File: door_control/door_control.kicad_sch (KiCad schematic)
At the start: 27 parts

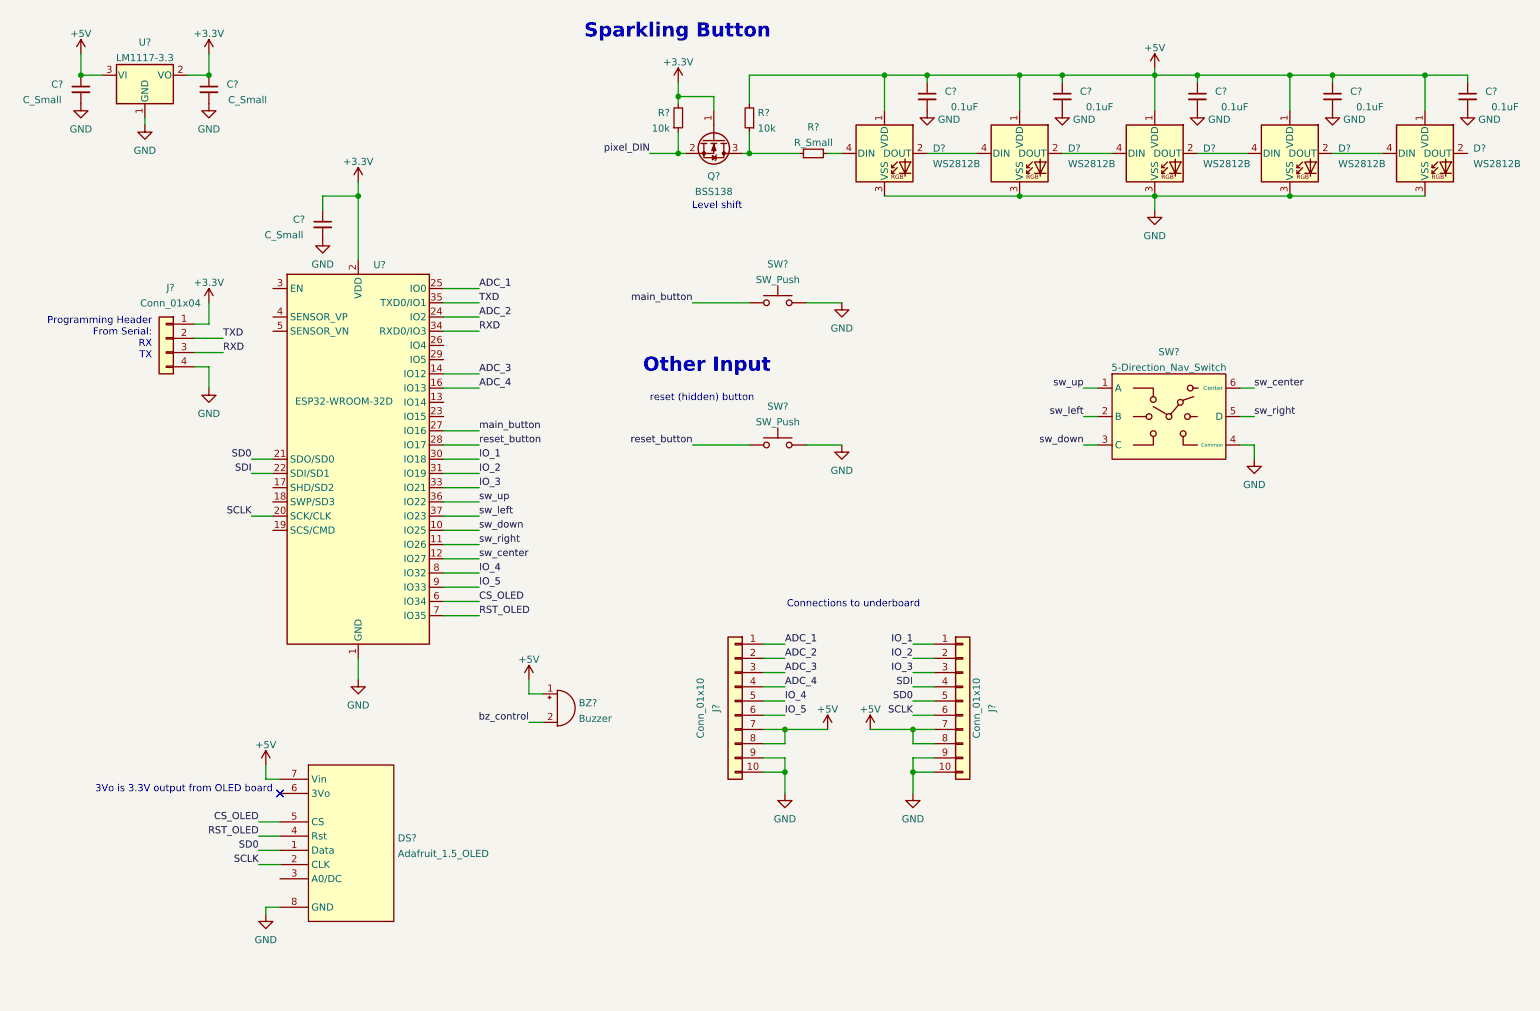
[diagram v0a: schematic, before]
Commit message: door control schematic update
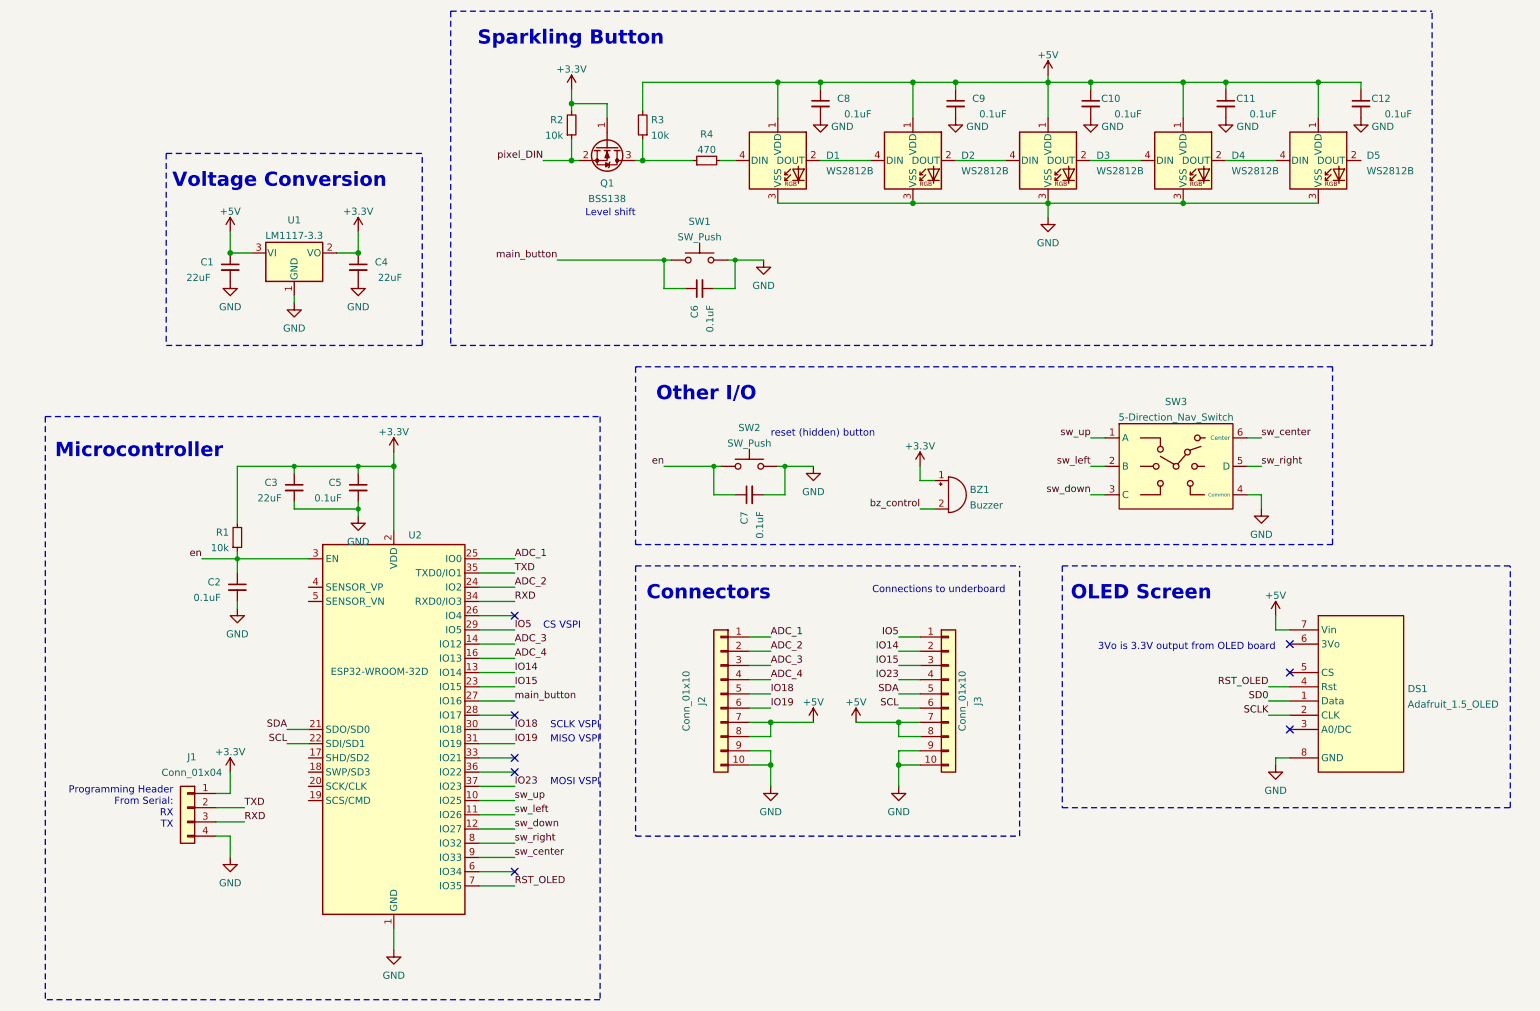
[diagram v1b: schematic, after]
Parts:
- added C2, C6, C7: 0.1uF, symbol Device:C_Small
- added C3: 22uF, symbol Device:C_Small
- added R1: 10k, symbol Device:R_Small
- C1, C4: renamed from C?; value C_Small -> 22uF
- C5: renamed from C?; value C_Small -> 0.1uF
- R4: renamed from R?; value R_Small -> 470
- gave numbers to parts that had none: 23
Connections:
- net +3V3: now also BZ1.1 (-), C3.1, R1.2
- net +5V: no longer BZ1.1 (-)
- net GND: now also C2.2, C3.2, C6.2, C7.2
- net SCLK: no longer J3.6 (Pin_6), U2.20 (SCK/CLK)
- net SD0: no longer J3.5 (Pin_5), U2.21 (SDO/SD0)
- net main_button: now also C6.1
- net sw_center: now also U2.9 (IO33); no longer U2.12 (IO27)
- net sw_down: now also U2.12 (IO27); no longer U2.10 (IO25)
- net sw_left: now also U2.11 (IO26); no longer U2.37 (IO23)
- net sw_right: now also U2.8 (IO32); no longer U2.11 (IO26)
- net sw_up: now also U2.10 (IO25); no longer U2.36 (IO22)
- net IO14: now reaches U2.13 (IO14)
- net IO14: now also J3.2 (Pin_2)
- net IO15: now reaches U2.23 (IO15)
- net IO15: now also J3.3 (Pin_3)
- net IO5: now reaches U2.29 (IO5)
- net IO5: now also J3.1 (Pin_1)
- net en: now reaches U2.3 (EN)
- net en: now also SW2.1, C2.1, C7.1, R1.1
- net CS_OLED: no longer names the net of U2.6 (IO34)
- net CS_OLED: no longer DS1.5 (CS)
- net IO_1 renamed IO18
- net IO18: now also J2.5 (Pin_5); no longer J3.1 (Pin_1)
- net IO_2 renamed IO19
- net IO19: now also J2.6 (Pin_6); no longer J3.2 (Pin_2)
- net IO_3: no longer names the net of U2.33 (IO21)
- net IO_3: no longer J3.3 (Pin_3)
- removed net IO_4: J2.5 (Pin_5), U2.8 (IO32)
- removed net IO_5: J2.6 (Pin_6), U2.9 (IO33)
- net SDI renamed IO23
- net IO23: now also U2.37 (IO23); no longer U2.22 (SDI/SD1)
- net reset_button: no longer names the net of U2.28 (IO17)
- net reset_button: no longer SW2.1
- new net SCL: J3.6 (Pin_6), U2.22 (SDI/SD1)
- new net SDA: J3.5 (Pin_5), U2.21 (SDO/SD0)
- no-connect marks 1 -> 8
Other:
- note added: "CS VSPI"
- note added: "Connectors"
- note added: "MISO VSPI"
- note added: "MOSI VSPI"
- note added: "Microcontroller"
- note added: "OLED Screen"
- note added: "Other I/O"
- note added: "SCLK VSPI"
- note added: "Voltage Conversion"
- note removed: "Other Input"
- moved on the sheet: BZ1, C1, C10, C11, C12, C4, C5, C8, C9, D1, D2, D3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
